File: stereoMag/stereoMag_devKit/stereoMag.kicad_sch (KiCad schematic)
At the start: 19 parts, among them J1 GameBoy_GamePak_CGB-002, J2 TSM-110-01-S-DH-LC, J6 microSD, SW1 SPDT_Slide_SMD_6.7x2.6mm, U1 W25Q16JVSS, U2 FM24C64B, U3 W25Q16JVSS

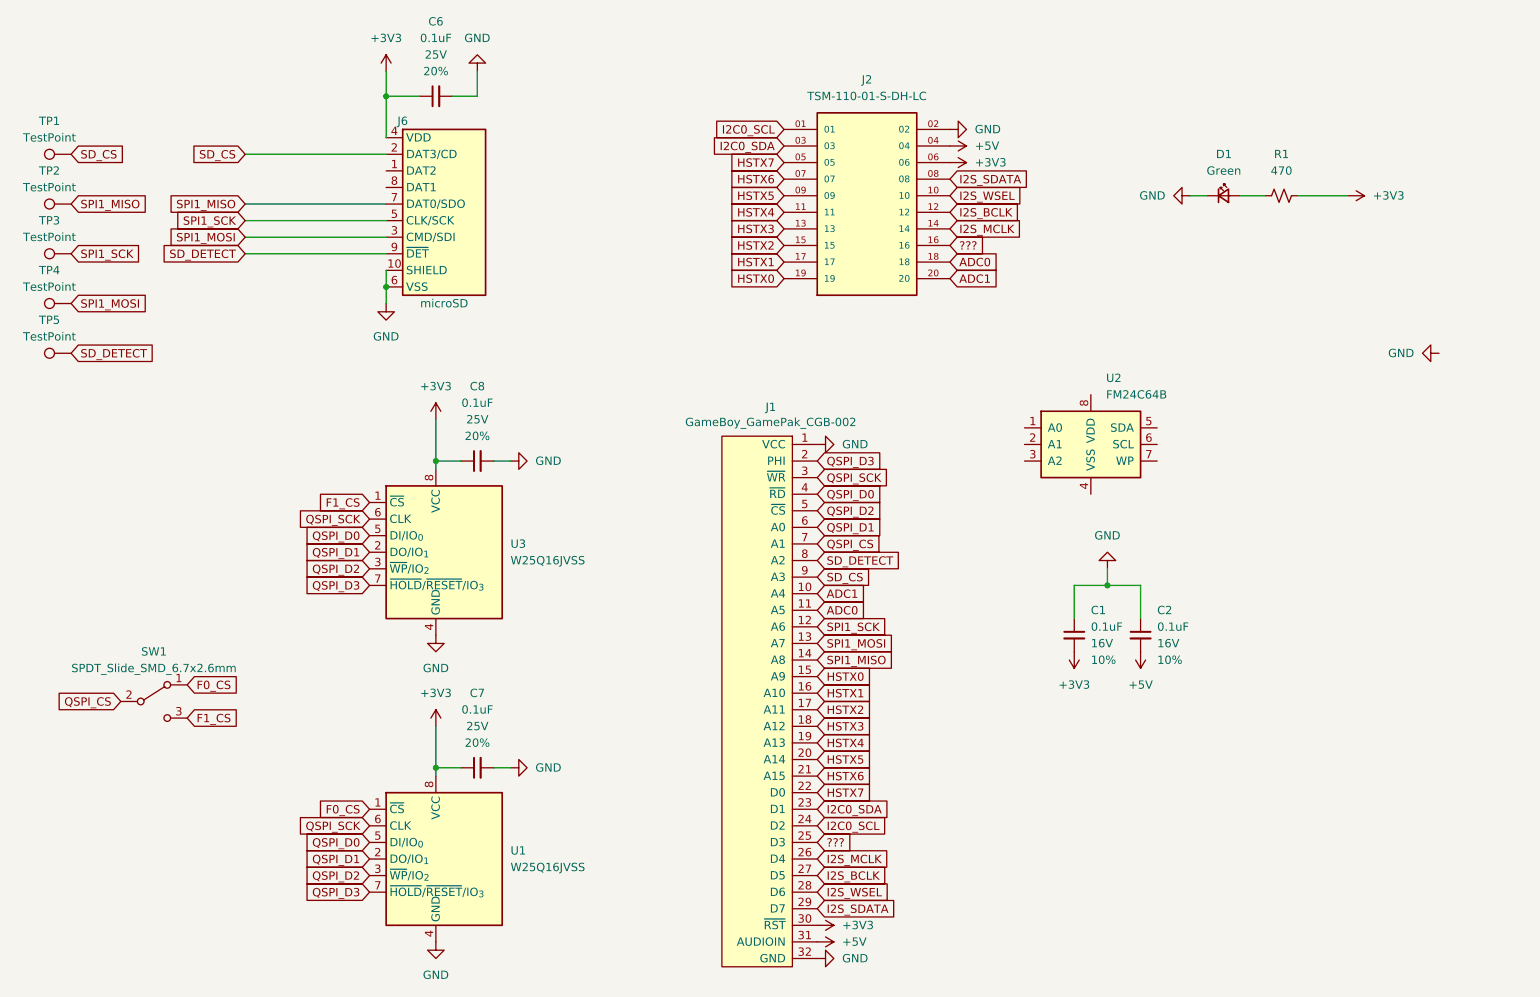
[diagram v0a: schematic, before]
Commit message: New thingies
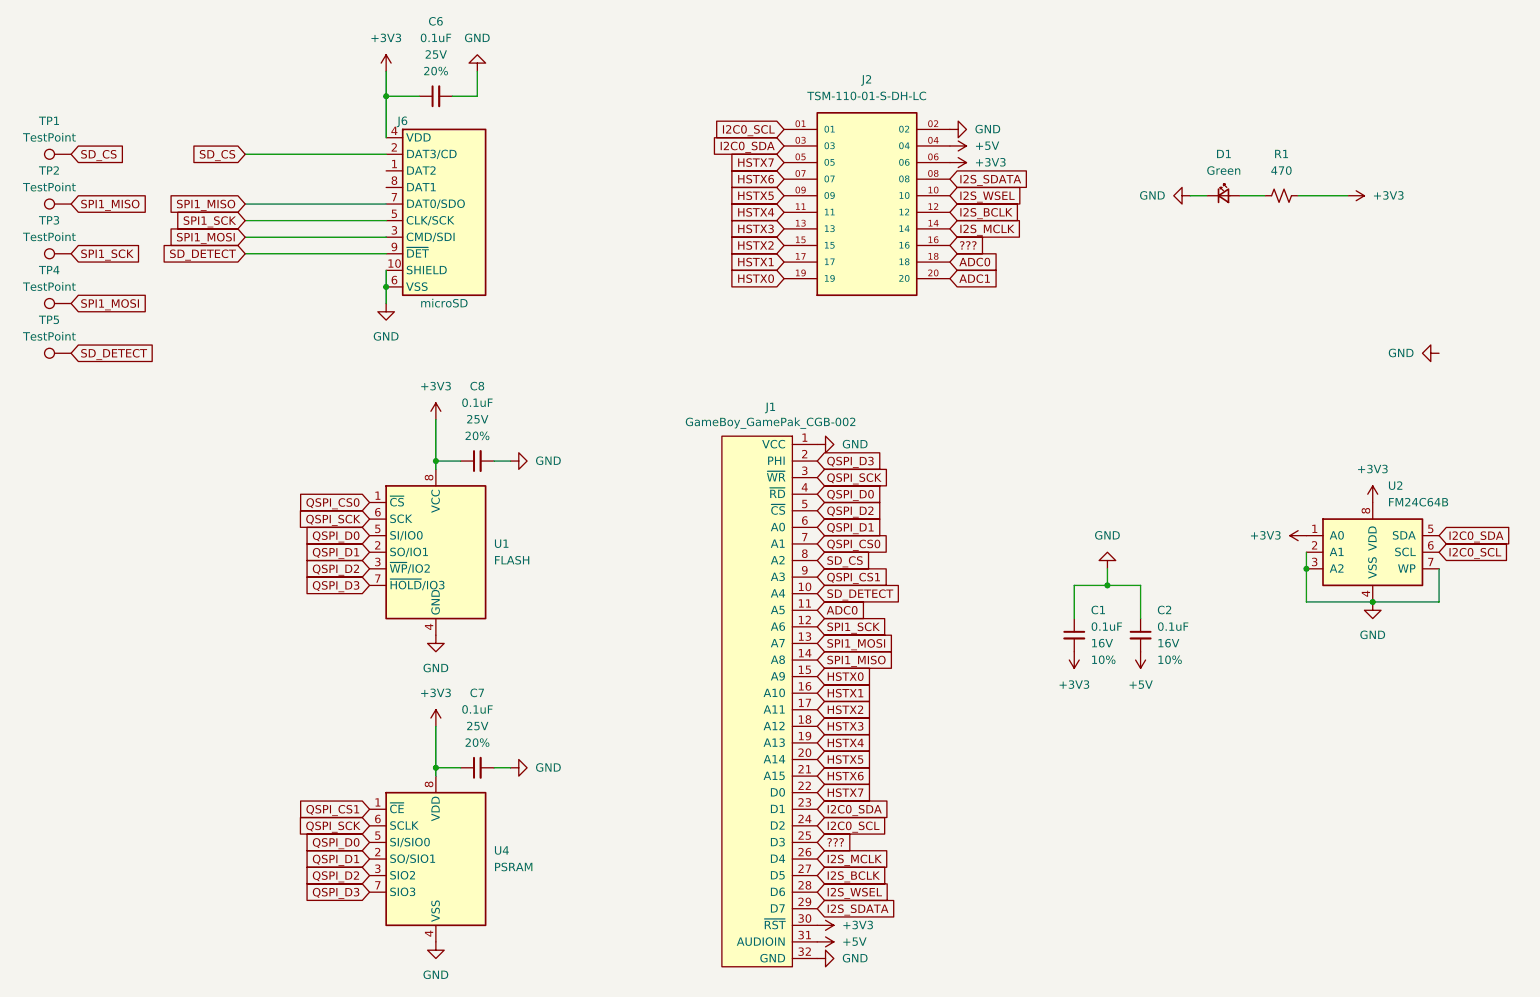
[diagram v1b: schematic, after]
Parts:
- removed SW1: SPDT_Slide_SMD_6.7x2.6mm, SparkFun-Switch:Slide_SPST_SMD_6.7x2.6mm, symbol SparkFun-Switch:SPDT_Slide_SMD_6.7x2.6mm
- removed U1, U3: W25Q16JVSS, Package_SO:SOIC-8_5.3x5.3mm_P1.27mm, symbol Memory_Flash:W25Q16JVSS
- added U1: FLASH, Package_SO:SOIC-8_3.9x4.9mm_P1.27mm, symbol Memory_Flash:AT25SF081-SSHD-X
- added U4: PSRAM, Package_SO:SOIC-8_3.9x4.9mm_P1.27mm, symbol Memory_RAM:APS1604M-3SQRx-SN
- C1, C2: footprint Capacitor_SMD:CP_Elec_5x3 -> Capacitor_SMD:C_1206_3216Metric
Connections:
- net +3V3: now also U2.1 (A0), U2.8 (VDD), U1.8 (VCC), U4.8 (VDD)
- net ADC1: no longer J1.10 (A4)
- net GND: now also U2.2 (A1), U2.3 (A2), U2.4 (VSS), U2.7 (WP), U1.4 (GND), U4.4 (VSS)
- net I2C0_SCL: now also U2.6 (SCL)
- net I2C0_SDA: now also U2.5 (SDA)
- net QSPI_D0: now also U1.5 (SI/IO0), U4.5 (SI/SIO0)
- net QSPI_D1: now also U1.2 (SO/IO1), U4.2 (SO/SIO1)
- net QSPI_D2: now also U1.3 (~{WP}/IO2), U4.3 (SIO2)
- net QSPI_D3: now also U1.7 (~{HOLD}/IO3), U4.7 (SIO3)
- net QSPI_SCK: now also U1.6 (SCK), U4.6 (SCLK)
- net SD_CS: now also J1.8 (A2); no longer J1.9 (A3)
- net SD_DETECT: now also J1.10 (A4); no longer J1.8 (A2)
- net QSPI_CS renamed QSPI_CS0
- net QSPI_CS0: now also U1.1 (~{CS})
- new net QSPI_CS1: J1.9 (A3), U4.1 (~{CE})
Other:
- moved on the sheet: U2
